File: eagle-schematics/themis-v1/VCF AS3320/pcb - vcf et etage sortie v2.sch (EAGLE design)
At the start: 38 parts

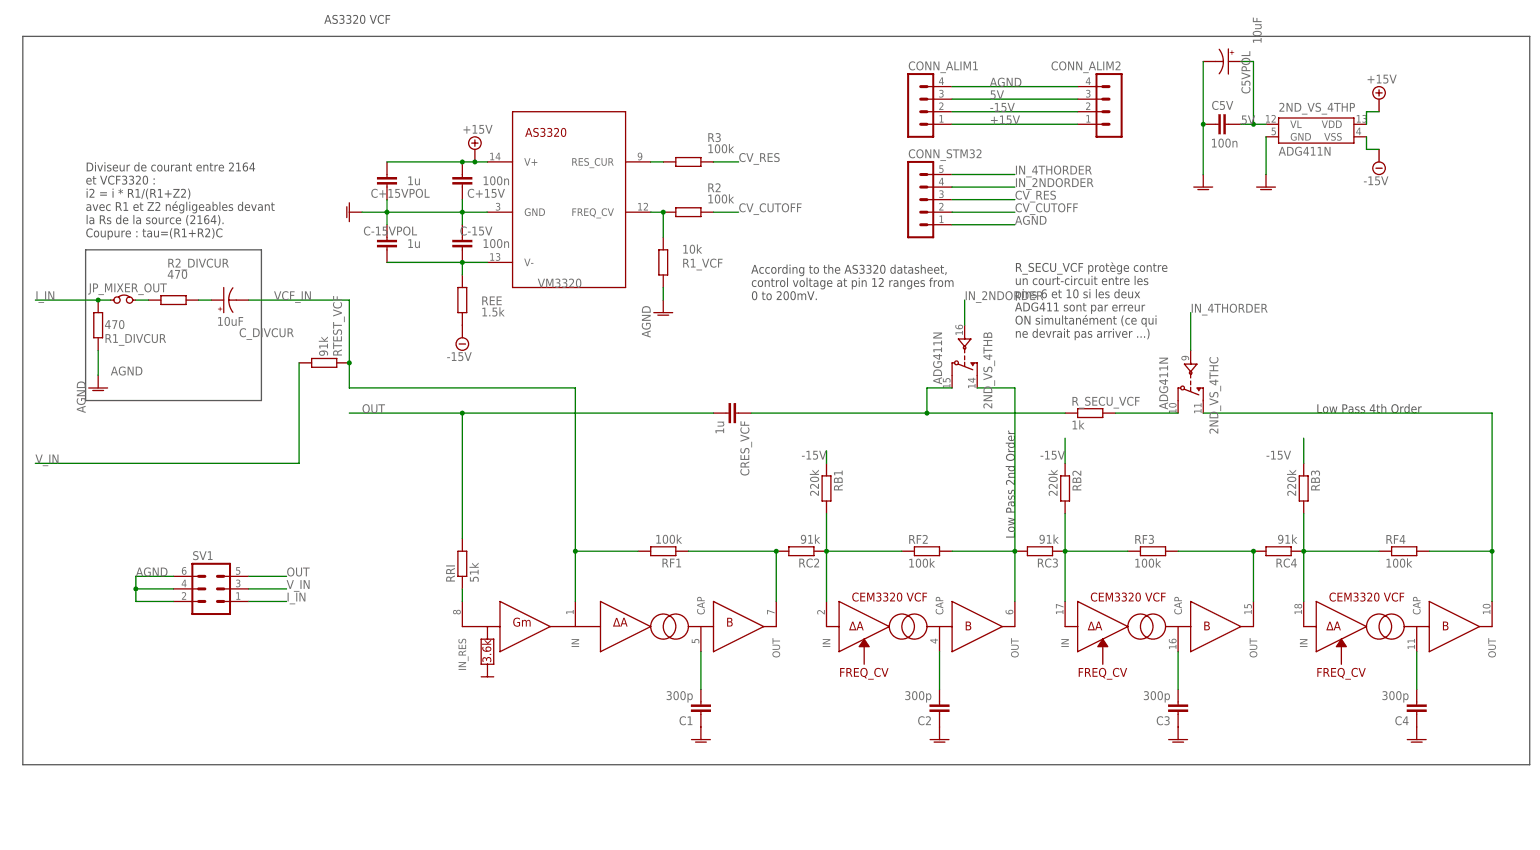
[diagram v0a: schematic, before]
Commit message: version 1 nouveau pcb vcf
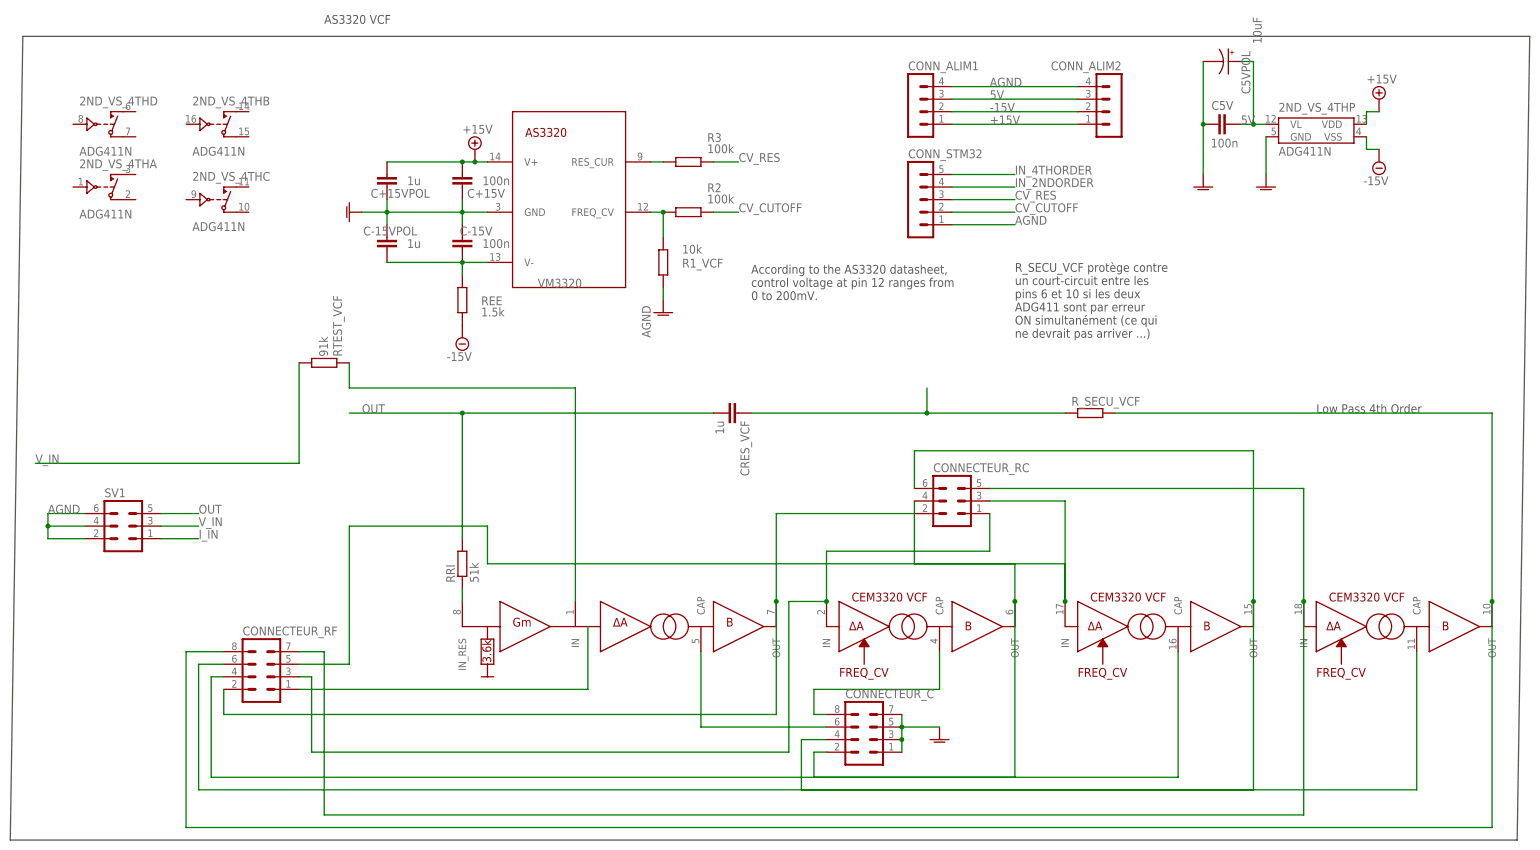
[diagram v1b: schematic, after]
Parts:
- removed C1, C2: 300p, rcl:C-EU050-024X044
- removed C3, C4: 300p, rcl:C-EU075-032X103
- removed C_DIVCUR: 10uF, SparkFun-Capacitors:10UF-POLAR-RADIAL-2.5MM-KIT-25V-20%
- removed JP_MIXER_OUT: JUMPER_WIRE, 6P1_EVB:JUMPER_WIRE
- removed R1_DIVCUR, R2_DIVCUR: 470, rcl:R-EU_0207/10
- removed RB1: 220k, rcl:R-EU_0207/10
- removed RB2: 220k, rcl:R-EU_0204/7
- removed RB3: 220k, rcl:R-EU_0204/5
- removed RC2, RC4: 91k, rcl:R-EU_0204/7
- removed RC3: 91k, rcl:R-EU_0204/5
- removed RF1, RF3: 100k, rcl:R-EU_0207/10
- removed RF2: 100k, rcl:R-EU_0204/5
- removed RF4: 100k, rcl:R-EU_0204/7
- added CONNECTEUR_C, CONNECTEUR_RF: (no value), con-lstb:MA04-2
- added CONNECTEUR_RC: (no value), con-lstb:MA03-2
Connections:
- removed net N$17: C3.2, VCFOTA$4.CAP
- removed net N$18: C2.2, VCFOTA$2.CAP
- removed net N$24: C4.2, VCFOTA$3.CAP
- removed net N$57: RC2.2, RF1.1, VCFOTA$1.OUT
- removed net N$62: RB1.2, RC2.1, RF2.1, VCFOTA$2.IN
- removed net N$65: 2ND_VS_4THB.S, RC3.2, RF2.2, VCFOTA$2.OUT
- removed net N$72: RB2.2, RC3.1, RF3.1, VCFOTA$4.IN
- removed net N$73: 2ND_VS_4THC.D, R_SECU_VCF.2
- removed net N$75: C_DIVCUR.+, R2_DIVCUR.1
- removed net N$79: JP_MIXER_OUT.2, R2_DIVCUR.2
- removed net N$82: RC4.2, RF3.2, VCFOTA$4.OUT
- removed net N$83: RB3.2, RC4.1, RF4.1, VCFOTA$3.IN
- new net N$1: CONNECTEUR_RF.1
- new net N$10: CONNECTEUR_RC.6, CONNECTEUR_RF.6, VCFOTA$4.OUT
- new net N$11: CONNECTEUR_RC.5, CONNECTEUR_RF.7, VCFOTA$3.IN
- new net N$2: CONNECTEUR_RC.2, CONNECTEUR_RF.2, VCFOTA$1.OUT
- new net N$3: CONNECTEUR_C.4, VCFOTA$3.CAP
- new net N$4: CONNECTEUR_C.2, VCFOTA$4.CAP
- new net N$6: CONNECTEUR_C.6, VCFOTA$1.CAP
- new net N$7: CONNECTEUR_RC.1, CONNECTEUR_RF.3, VCFOTA$2.IN
- new net N$8: CONNECTEUR_RC.4, CONNECTEUR_RF.4, VCFOTA$2.OUT
- new net N$9: CONNECTEUR_RC.3, CONNECTEUR_RF.5, VCFOTA$4.IN
- net -15V: no longer RB1.1, RB2.1, RB3.1
- net AGND: now also CONNECTEUR_C.1, CONNECTEUR_C.3, CONNECTEUR_C.5, CONNECTEUR_C.7; no longer C1.1, C2.1, C3.1, C4.1, R1_DIVCUR.2
- net IN_2NDORDER: no longer 2ND_VS_4THB.IN
- net IN_4THORDER: no longer 2ND_VS_4THC.IN
- net I_IN: no longer JP_MIXER_OUT.1, R1_DIVCUR.1
- net N$5: now also CONNECTEUR_C.8, VCFOTA$2.CAP; no longer C1.2, VCFOTA$1.CAP
- net N$58: no longer 2ND_VS_4THB.D
- net N$69: now also CONNECTEUR_RF.8, R_SECU_VCF.2; no longer 2ND_VS_4THC.S, RF4.2
- net VCF_IN: no longer C_DIVCUR.-, RF1.2
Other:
- note removed: "Diviseur de courant entre 2164 et VCF3320 : i2 = i * R1/(R1+Z2) avec R1 et Z2 négligeables devant la Rs de la source (2164). Coupure : tau=(R1+R2)C"
- note removed: "Low Pass 2nd Order"
- moved on the sheet: 2ND_VS_4THB, 2ND_VS_4THC, SV1
